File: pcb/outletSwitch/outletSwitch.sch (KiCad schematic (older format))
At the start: 15 parts

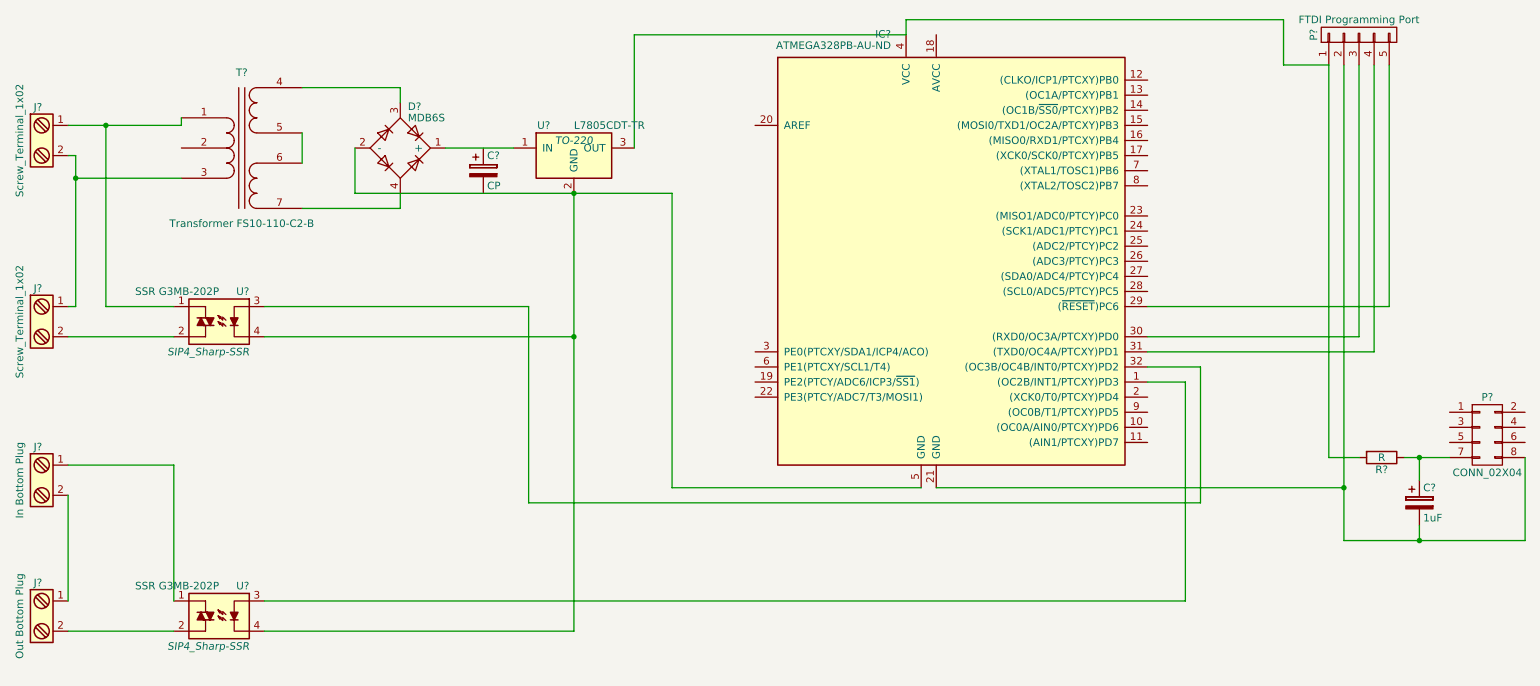
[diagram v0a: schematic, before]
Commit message: added js that alerts the status of hackpgh's door
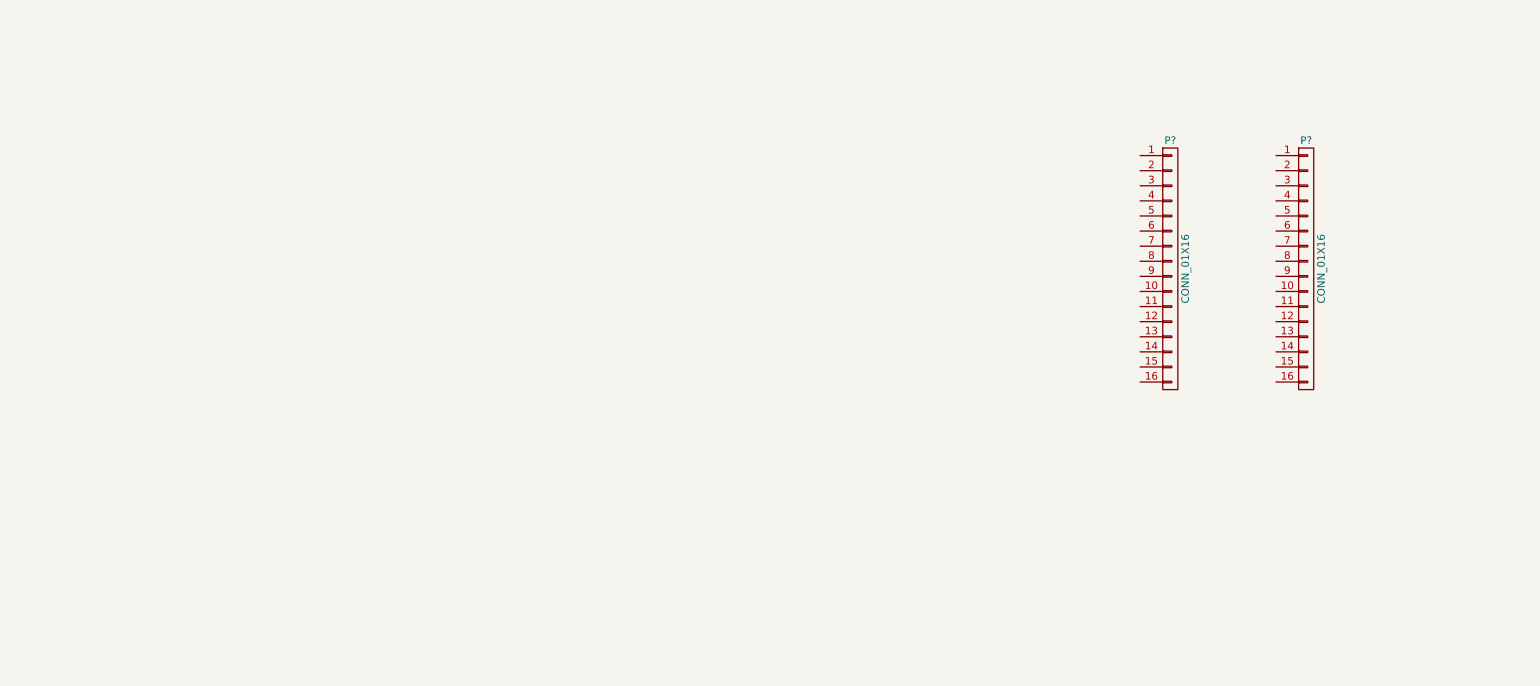
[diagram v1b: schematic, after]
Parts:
- removed C?: CP, symbol CP
- removed C?: 1uF, symbol CP
- removed D?: MDB6S, symbol D_Bridge_+-AA
- removed IC?: ATMEGA328PB-AU-ND, Housings_QFP:TQFP-32_7x7mm_Pitch0.8mm, symbol ATMEGA328PB-A
- removed J? (x2): Screw_Terminal_1x02, symbol Screw_Terminal_1x02
- removed J?: In Bottom Plug, symbol Screw_Terminal_1x02
- removed J?: Out Bottom Plug, symbol Screw_Terminal_1x02
- removed P?: FTDI Programming Port, symbol CONN_01X05
- removed P?: CONN_02X04, symbol CONN_02X04
- removed R?: R, symbol R
- removed T?: Transformer FS10-110-C2-B, symbol Transformer_SP_2S
- removed U?: L7805CDT-TR, TO-220, symbol LM7805CT
- removed U? (x2): SSR G3MB-202P, SIP4_Sharp-SSR, symbol S102S01
- added P? (x2): CONN_01X16, symbol CONN_01X16
